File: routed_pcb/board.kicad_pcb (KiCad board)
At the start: 2 copper layers, 100 x 100 mm, 29 parts

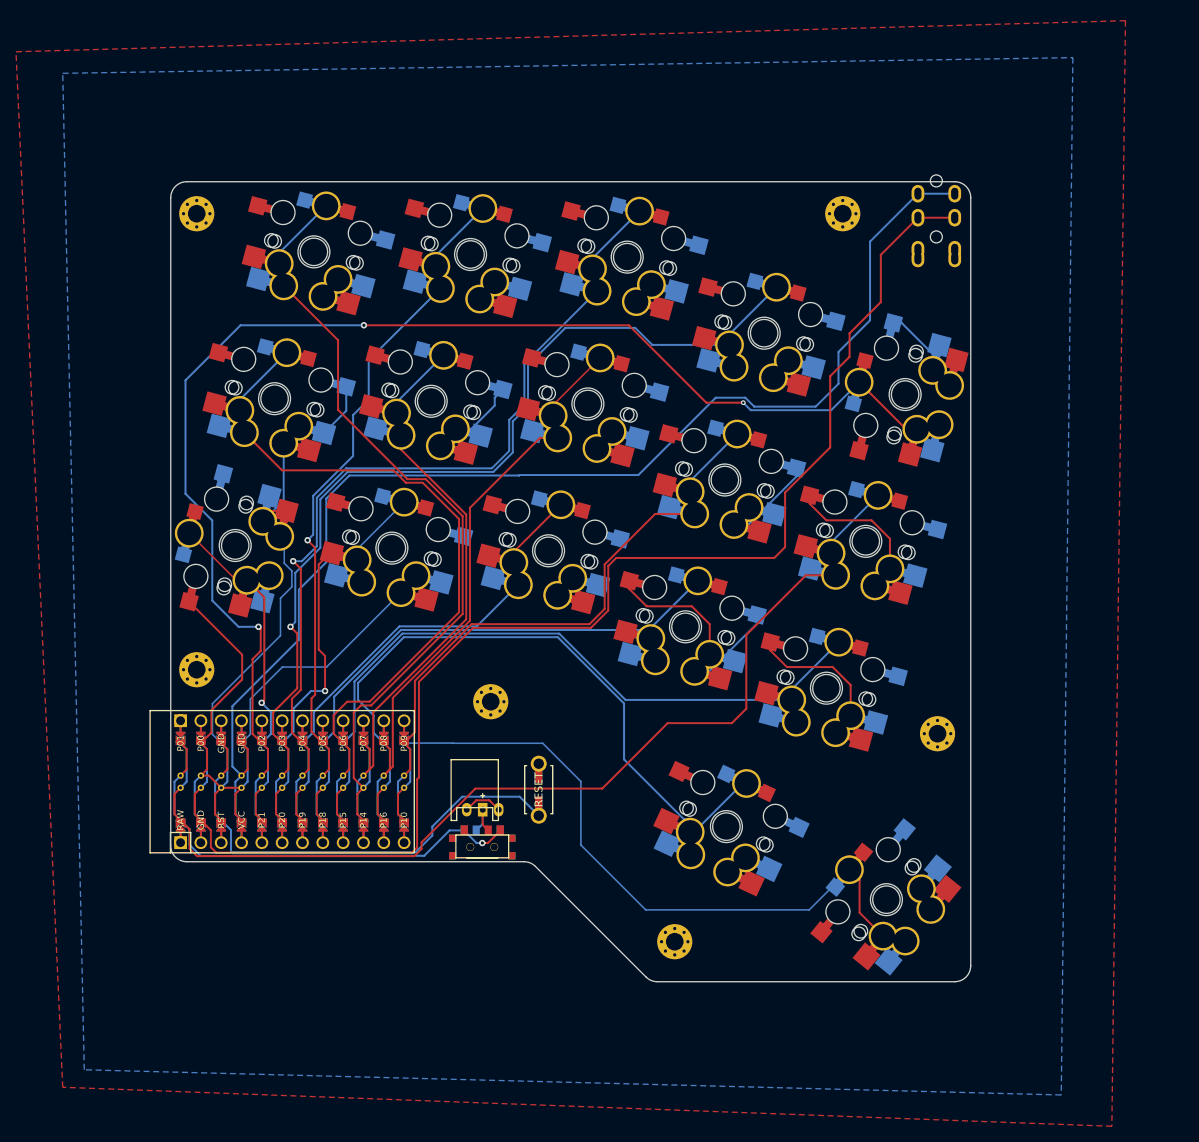
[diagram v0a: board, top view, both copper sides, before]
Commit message: routed new pcb
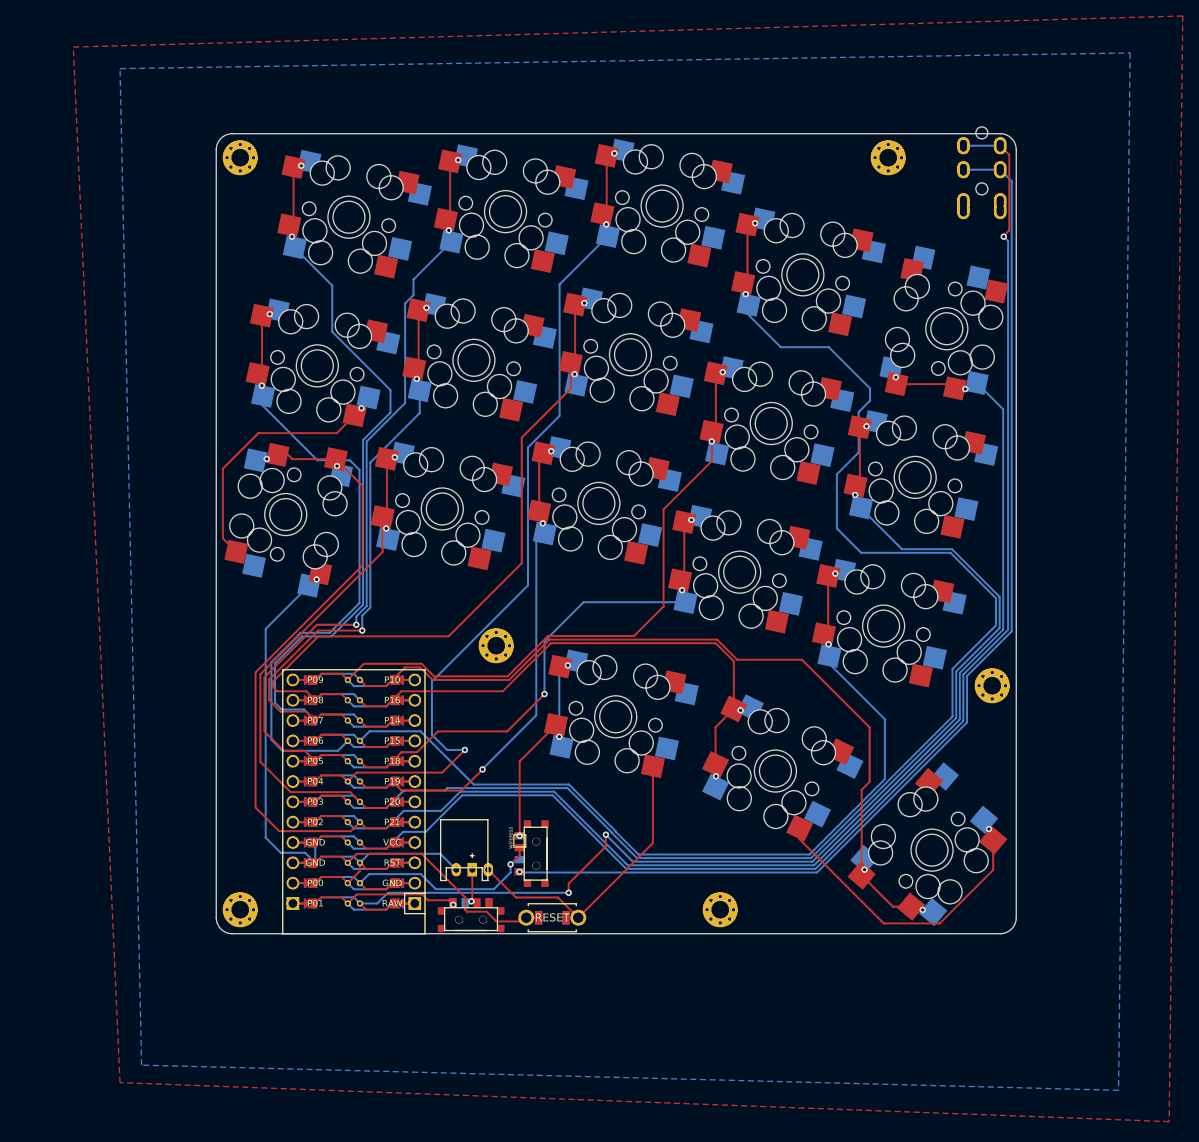
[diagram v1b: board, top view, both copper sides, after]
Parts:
- removed the ? at (108.7, 153.0)
- removed S1, S10, S11, S12, S13, S14, S15, S16, S17, S2, S3, S4, S5, S6, S7, S8, S9: , Library:key-switches
- removed _2: , Library:JST_PH_S2B-PH-K_02x2.00mm_Angled
- removed _3, _4, _5: , Library:MountingHole_2.2mm_M2_Pad_Via
- added ?: , Button_Switch_SMD:SW_SPST_B3U-1000P, F.Cu at (110.3, 169.0)
- added SW1: , key-switches, F.Cu at (77.0, 118.6)
- added SW10: , key-switches, F.Cu at (133.8, 125.8)
- added SW11: , key-switches, F.Cu at (137.7, 107.2)
- added SW12: , key-switches, F.Cu at (141.7, 88.6)
- added SW13: , key-switches, F.Cu at (151.8, 132.5)
- added SW14: , key-switches, F.Cu at (155.7, 114.0)
- added SW15: , key-switches, F.Cu at (159.7, 95.4)
- added SW16: , key-switches, F.Cu at (118.3, 143.9)
- added SW17: , key-switches, F.Cu at (138.2, 150.7)
- added SW18: , key-switches, F.Cu at (157.8, 160.6)
- added SW2: , key-switches, F.Cu at (81.0, 100.0)
- added SW3: , key-switches, F.Cu at (84.9, 81.4)
- added SW4: , key-switches, F.Cu at (96.6, 117.9)
- added SW5: , key-switches, F.Cu at (100.5, 99.3)
- added SW6: , key-switches, F.Cu at (104.5, 80.7)
- added SW7: , key-switches, F.Cu at (116.2, 117.2)
- added SW8: , key-switches, F.Cu at (120.1, 98.6)
- added SW9: , key-switches, F.Cu at (124.1, 80.0)
- added T2: , E73:SPDT_C128955, F.Cu at (108.3, 161.0)
- added _10: , MountingHole_2.2mm_M2_Pad_Via, F.Cu at (131.3, 168.0)
- added _11: , MountingHole_2.2mm_M2_Pad_Via, F.Cu at (103.3, 135.0)
- added _12: , MountingHole_2.2mm_M2_Pad_Via, F.Cu at (71.3, 168.0)
- added _9: , MountingHole_2.2mm_M2_Pad_Via, F.Cu at (165.3, 140.0)
- B1: footprint Library:ResetSW -> kbd:ResetSW
- MCU1: footprint Library:ProMicro -> ProMicro
- T1: footprint Library:SPDT_C128955 -> E73:SPDT_C128955
- TRRS1: footprint Library:TRRS-PJ-320A-dual -> TRRS-PJ-320A-dual
- _6: footprint Library:MountingHole_2.2mm_M2_Pad_Via -> JST_PH_S2B-PH-K_02x2.00mm_Angled
- _7, _8: footprint Library:MountingHole_2.2mm_M2_Pad_Via -> MountingHole_2.2mm_M2_Pad_Via
- moved _8 107.6 mm to (152.3, 74.0)
- moved _7 74.9 mm to (71.3, 74.0)
- moved _6 26.9 mm to (100.3, 163.0), turned to 180 degrees
- moved B1 16.1 mm to (110.3, 169.0), turned to 180 degrees
- moved T1 9.19 mm to (100.2, 169.2)
- moved TRRS1 8.27 mm to (166.3, 69.3)
- moved MCU1 7.79 mm to (85.5, 153.2), turned to 90 degrees
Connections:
- MCU1 pad 23: Switch18 -> P0
- T1 pad 1: (no net) -> RAW
- T1 pad 3: RAW -> (no net)
- TRRS1 pad 3: Switch18 -> trrs_data
- _6 pad 1: (no net) -> Bplus
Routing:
- net Switch18: track 159.7 -> 0.00 mm
- net trrs_data: track 0.00 -> 140.4 mm, vias 0 -> 1
- net matrix_index_top: track 109.9 -> 174.5 mm, vias 1 -> 2
- net matrix_pinky_bottom: track 36.2 -> 78.0 mm, vias 1 -> 2
- net GND: track 207.1 -> 169.6 mm, vias 0 -> 3
- net RAW: track 45.6 -> 14.2 mm
- net thumb_inner: track 0.00 -> 30.4 mm, vias 0 -> 3
- net matrix_inner_bottom: track 78.5 -> 107.5 mm, vias 0 -> 2
- net P0: track 0.00 -> 25.9 mm, vias 0 -> 1
- net matrix_inner_home: track 115.2 -> 140.7 mm, vias 0 -> 4
- net matrix_ring_bottom: track 40.6 -> 64.2 mm, vias 1 -> 2
- net matrix_middle_home: track 62.2 -> 84.2 mm, vias 0 -> 2
- net VCC: track 143.3 -> 165.2 mm, vias 0 -> 1
- net matrix_ring_top: track 74.5 -> 94.5 mm, vias 1 -> 3
- net thumb_reachy: track 81.1 -> 99.5 mm, vias 0 -> 2
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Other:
- outline, holes or cut-outs redrawn
- board text added: "wired"
- board text added: "wireless"
- board text added: "口"
